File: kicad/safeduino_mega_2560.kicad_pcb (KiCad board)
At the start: 4 copper layers, 134.5 x 63.9 mm, 130 parts, among them X1 USB

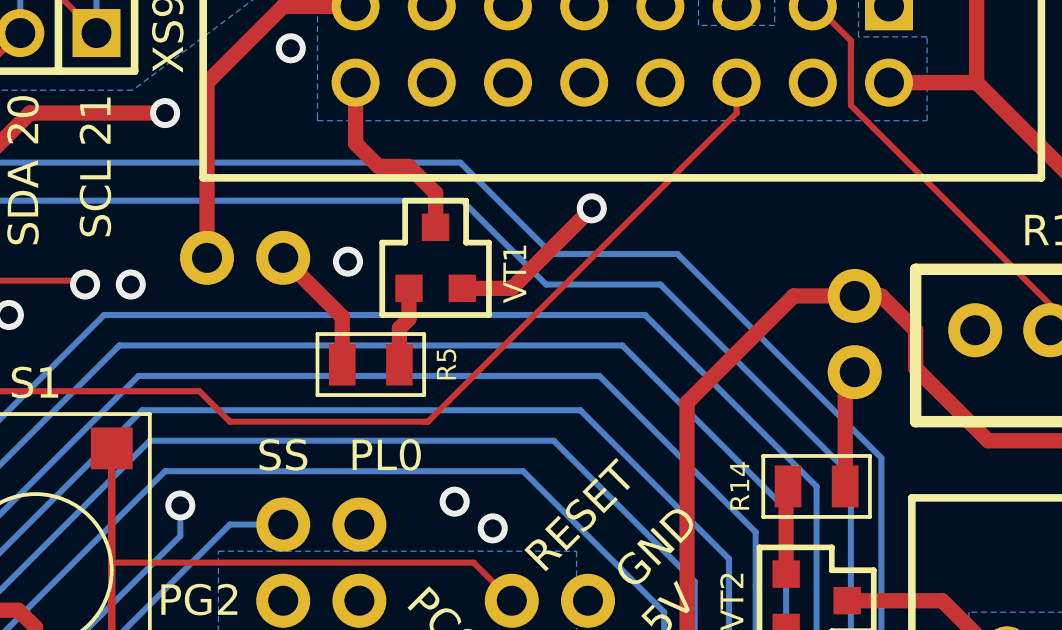
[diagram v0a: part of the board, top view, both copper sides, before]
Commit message: Продолжил переделывать проект.
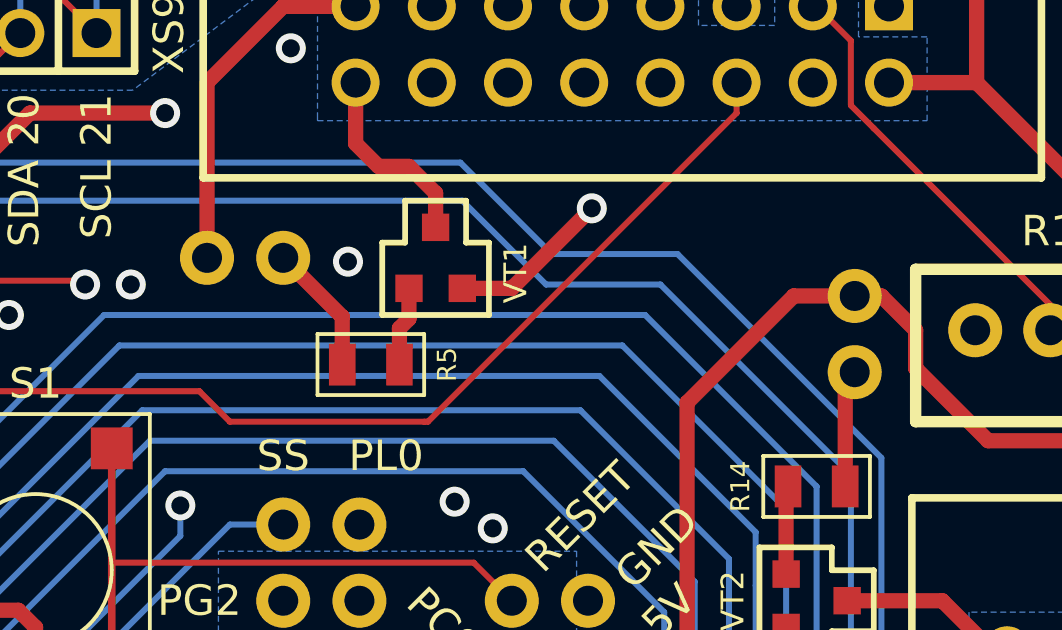
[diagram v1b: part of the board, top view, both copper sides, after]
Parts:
- XP16, XP20, XP21, XP26, XP27, XP28, XP29, XP32, XP36, XP37, XP38, XP39, XP40, XP41, XP42, XP48, XP53, XP54, XP55, XP56, XP57, XP58, XP59, XP60, XP61, XP62, XP65, XP67, XP68, XP7: footprint 1_pin -> IWconnectors:1_pin
